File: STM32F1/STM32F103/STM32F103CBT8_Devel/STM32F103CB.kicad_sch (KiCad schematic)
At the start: 24 parts, among them SW2 SW_DIP_x02

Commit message: Update MPNS and check
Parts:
- U?: Manufacturer STM32F103CBT7 -> STM32F103CBT6; mpn STM32F103CBT7 -> STM32F103CBT6
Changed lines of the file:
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@@
 			)
 		)
-		(property "Manufacturer" "STM32F103CBT7"
+		(property "Manufacturer" "STM32F103CBT6"
 			(at 49.53 81.28 0)
 			(effects
@@
 			)
 		)
-		(property "mpn" "STM32F103CBT7"
+		(property "mpn" "STM32F103CBT6"
 			(at 49.53 81.28 0)
 			(effects

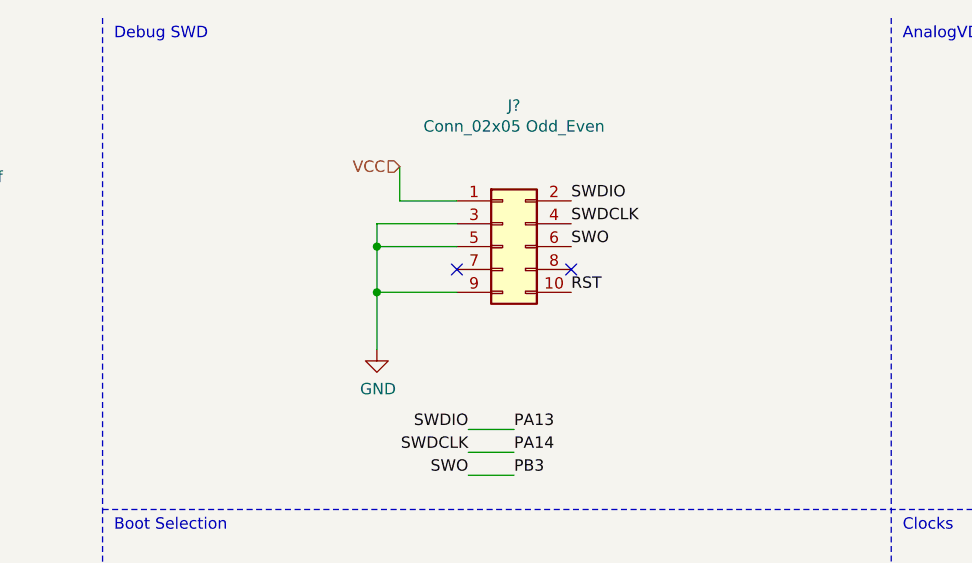
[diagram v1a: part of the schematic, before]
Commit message: 6Pin conector debug
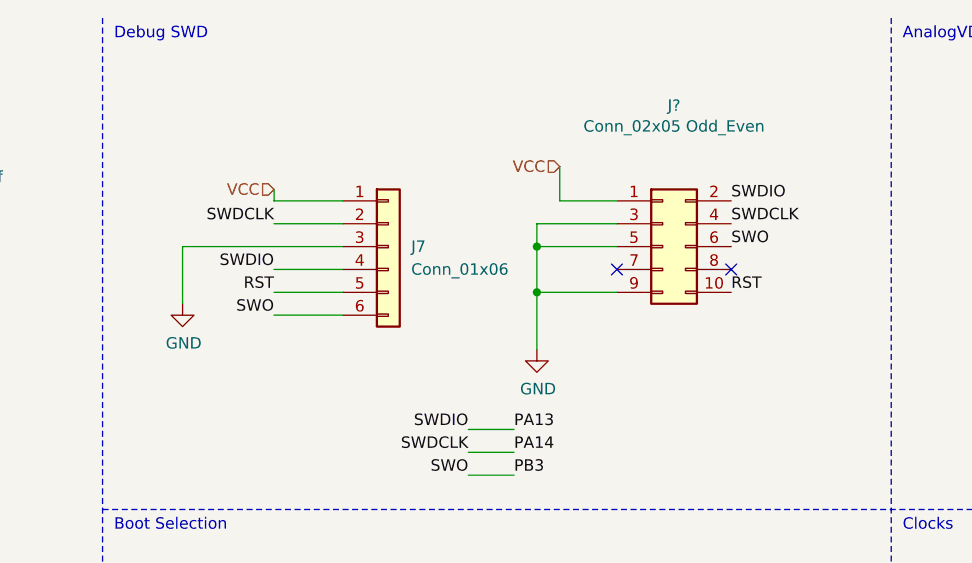
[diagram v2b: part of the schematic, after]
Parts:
- added J7: Conn_01x06, Connector_PinHeader_2.54mm:PinHeader_1x06_P2.54mm_Vertical, symbol Connector_Generic:Conn_01x06
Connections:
- net GND: now also J7.3 (Pin_3)
- net NRST: now also J7.5 (Pin_5)
- net PA13: now also J7.4 (Pin_4)
- net PA14: now also J7.2 (Pin_2)
- net PB3: now also J7.6 (Pin_6)
- net VCC: now also J7.1 (Pin_1)
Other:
- moved on the sheet: J?
